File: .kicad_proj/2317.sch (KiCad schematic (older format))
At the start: 1 part, among them U1 ATmega328-PU

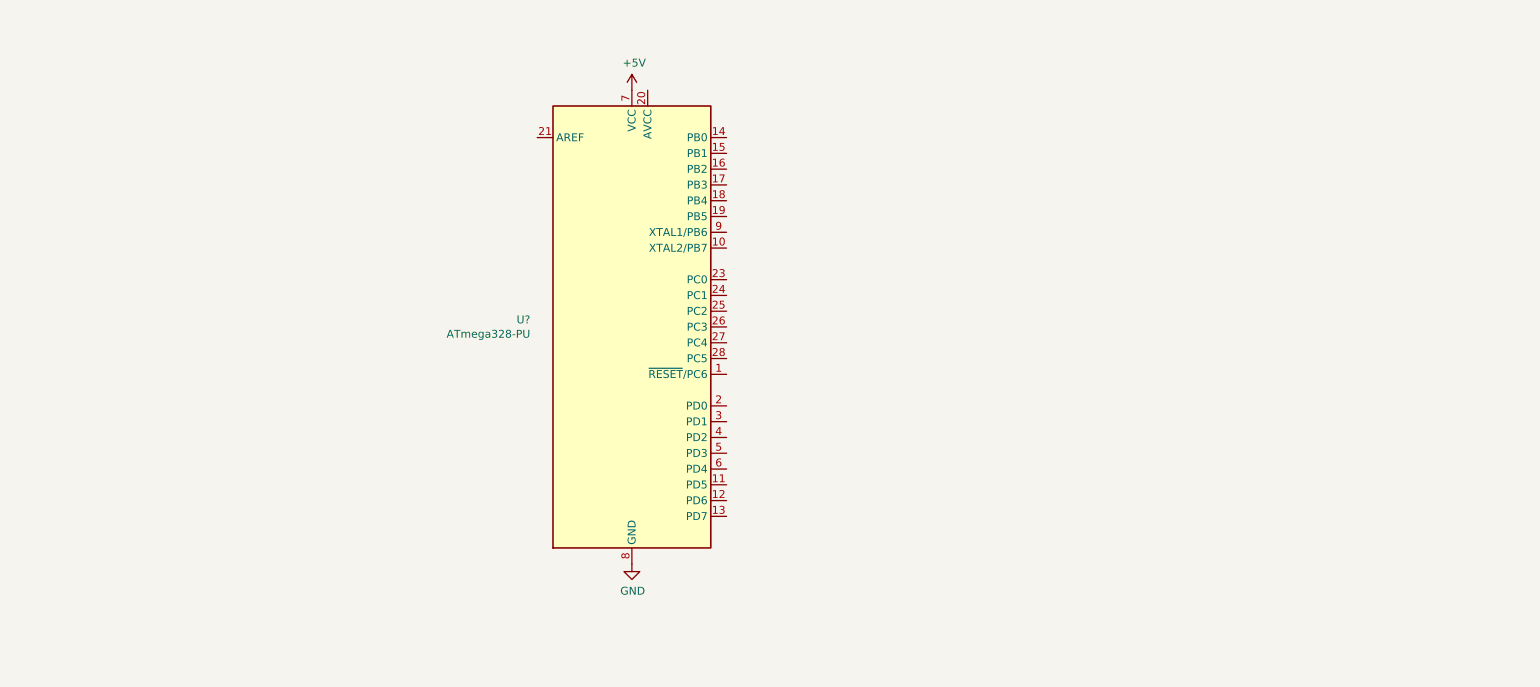
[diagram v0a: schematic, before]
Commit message: Add schematic 17
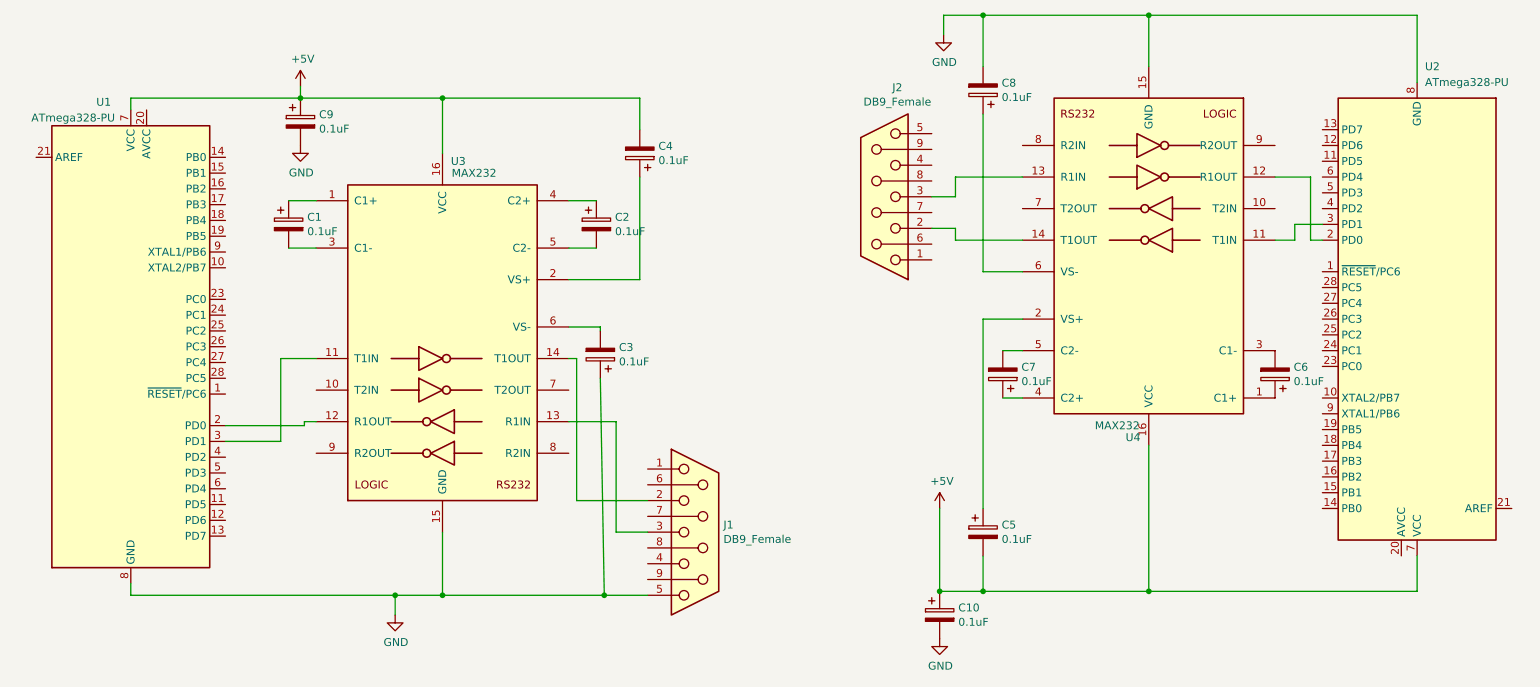
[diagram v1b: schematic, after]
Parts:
- added C1, C10, C2, C3, C4, C5, C6, C7, C8, C9: 0.1uF, symbol Device:CP
- added J1, J2: DB9_Female, symbol Connector:DB9_Female
- added U1: ATmega328-PU, Package_DIP:DIP-28_W7.62mm, symbol MCU_Microchip_ATmega:ATmega328-PU
- added U3, U4: MAX232, symbol Interface_UART:MAX232
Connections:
- net +5V: now also C10.1, C4.2, C5.2, C9.1, U1.7 (VCC), U3.16 (VCC), U4.16 (VCC)
- net GND: now also C10.2, C3.1, C8.2, C9.2, J1.5, U1.22 (GND), U1.8 (GND), U3.15 (GND), U4.15 (GND)
- net at U1.2 (PD0): now also U4.12 (R1OUT)
- net at U1.3 (PD1): now also U4.11 (T1IN)
- new net: C1.1, U3.1 (C1+)
- new net: U1.3 (PD1), U3.11 (T1IN)
- new net: U1.2 (PD0), U3.12 (R1OUT)
- new net: J1.3, U3.13 (R1IN)
- new net: J1.2, U3.14 (T1OUT)
- new net: C4.1, U3.2 (VS+)
- new net: C1.2, U3.3 (C1-)
- new net: C2.1, U3.4 (C2+)
- new net: C2.2, U3.5 (C2-)
- new net: C3.2, U3.6 (VS-)
- new net: C6.1, U4.1 (C1+)
- new net: J2.3, U4.13 (R1IN)
- new net: J2.2, U4.14 (T1OUT)
- new net: C5.1, U4.2 (VS+)
- new net: C6.2, U4.3 (C1-)
- new net: C7.1, U4.4 (C2+)
- new net: C7.2, U4.5 (C2-)
- new net: C8.1, U4.6 (VS-)
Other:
- moved on the sheet: U2
